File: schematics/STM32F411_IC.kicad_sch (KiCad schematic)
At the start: 24 parts

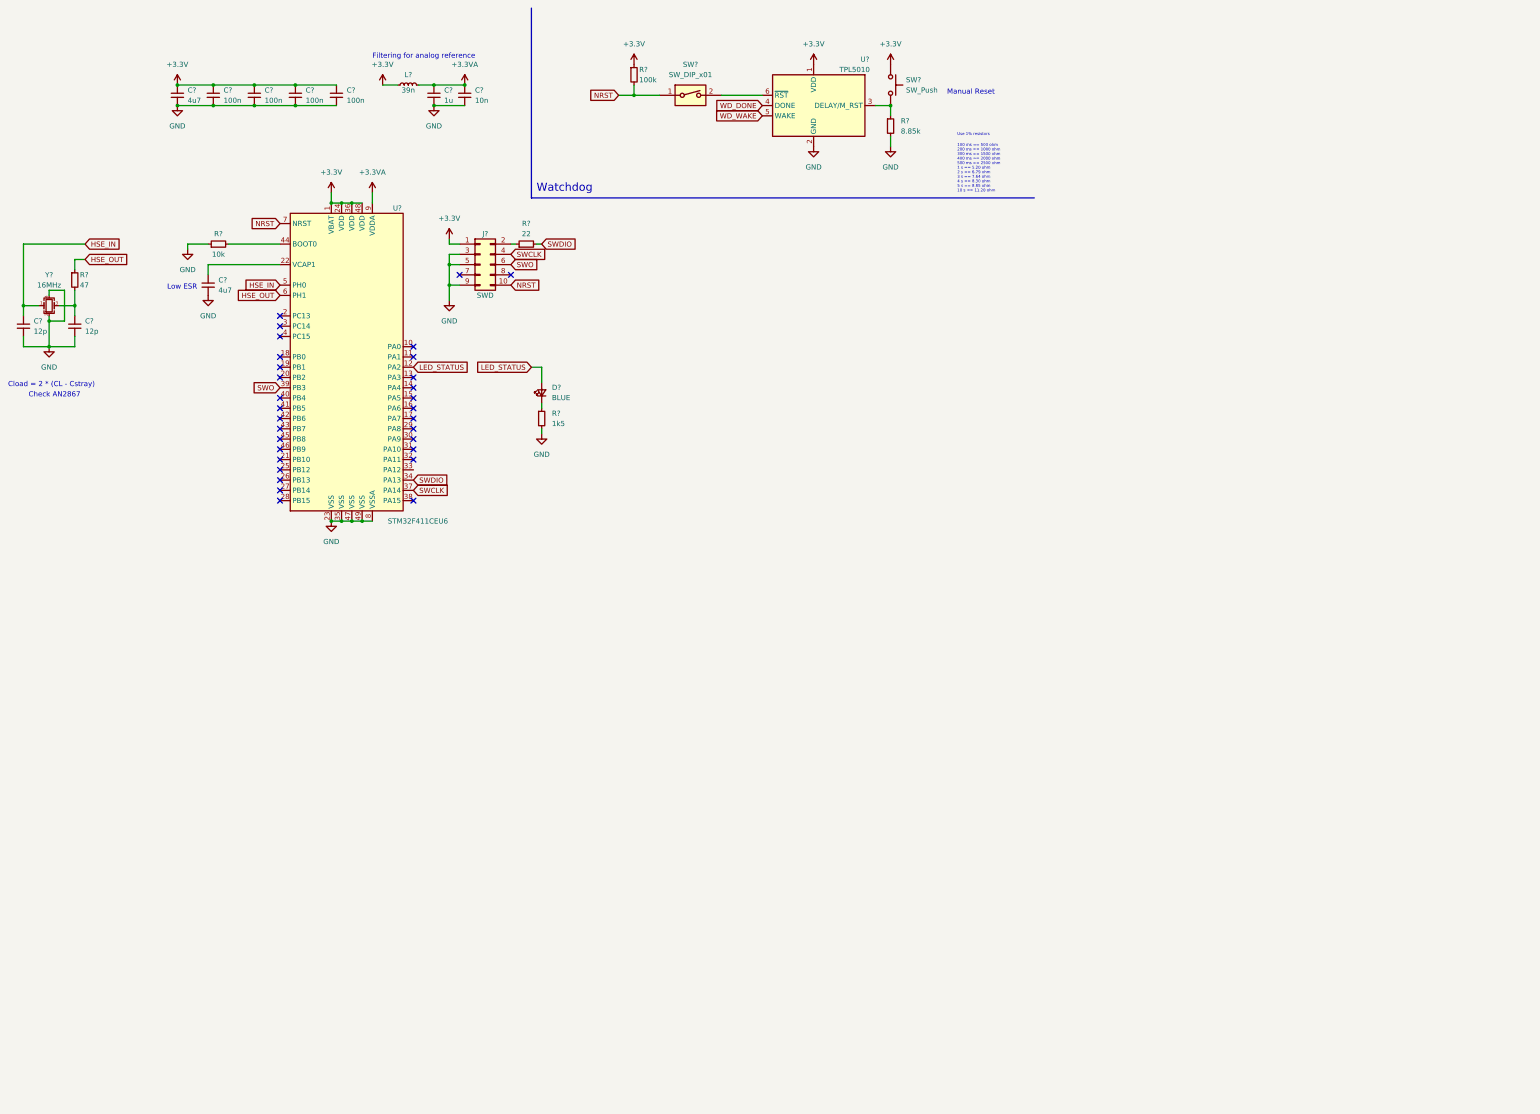
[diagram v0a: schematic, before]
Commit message: Add files via upload
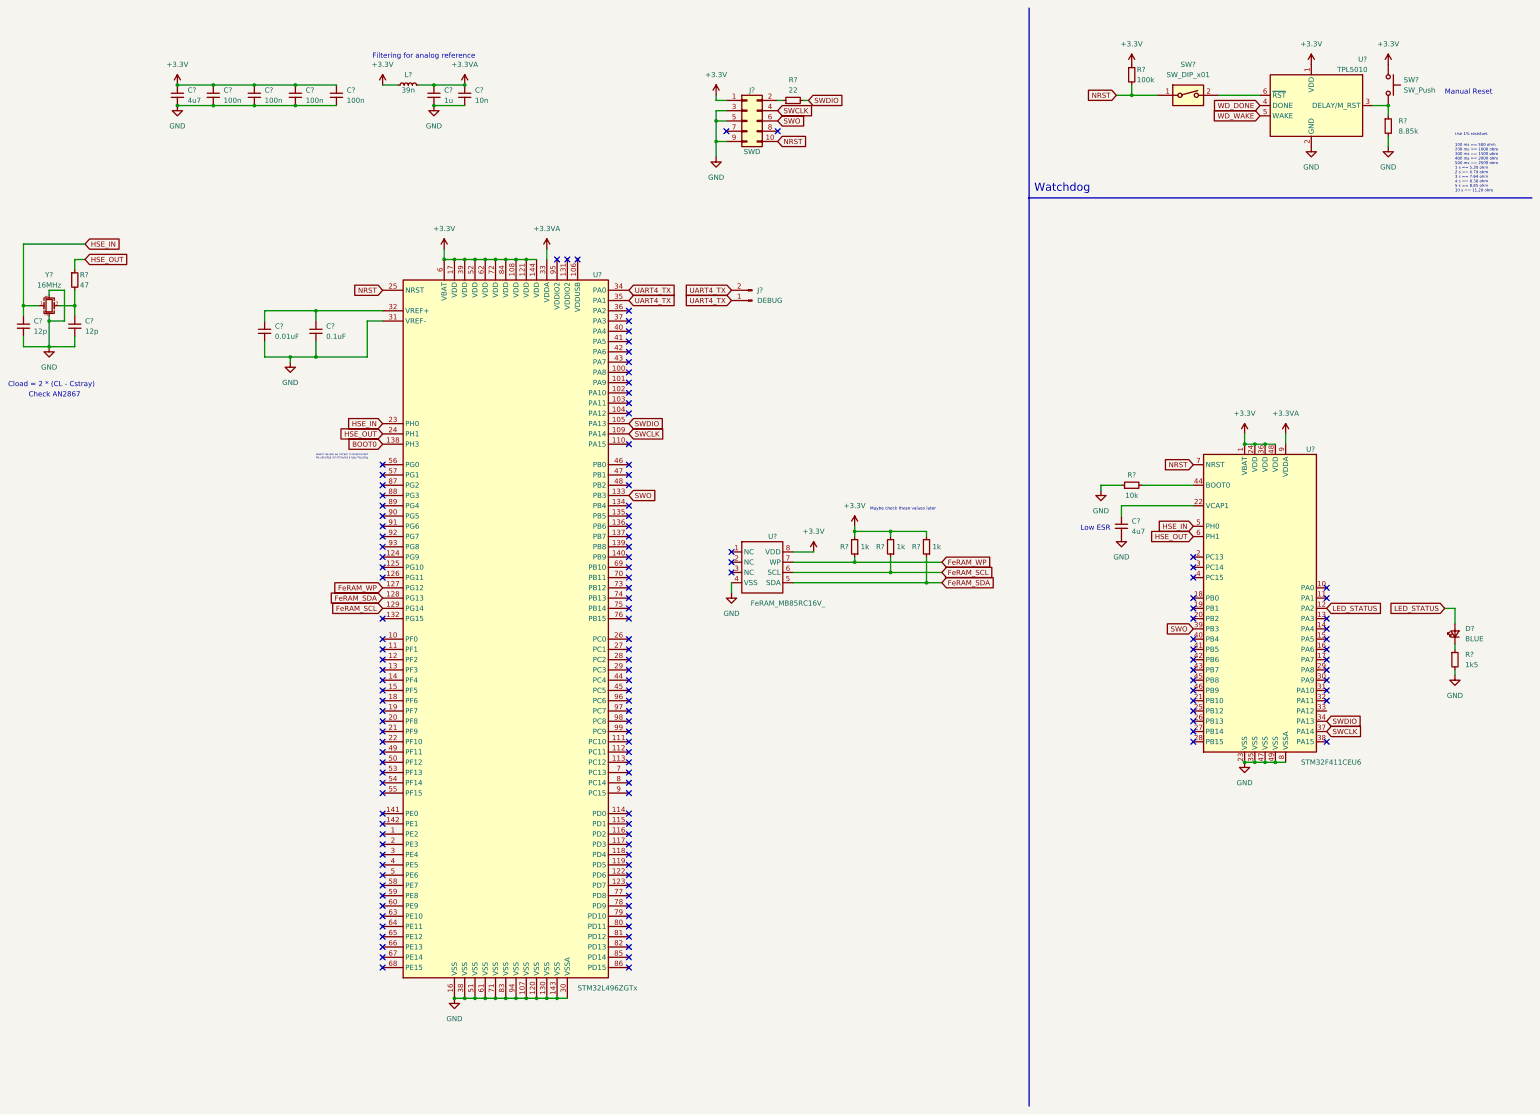
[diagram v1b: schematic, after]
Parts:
- added C?: 0.01uF, symbol Device:C_Small
- added C?: 0.1uF, symbol Device:C_Small
- added J?: DEBUG, symbol Connector:Conn_01x02_Male
- added R? (x3): 1k, symbol Device:R_Small
- added U?: STM32L496ZGTx, Package_QFP:LQFP-144_20x20mm_P0.5mm, symbol MCU_ST_STM32L4:STM32L496ZGTx
- added U?: FeRAM_MB85RC16V_, symbol MyKiCadLibrairy:FeRAM_MB85RC16V_
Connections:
- net +3.3V: now also R?.2, R?.2, R?.2, U?.108 (VDD), U?.121 (VDD), U?.144 (VDD), U?.17 (VDD), U?.39 (VDD), U?.52 (VDD), U?.6 (VBAT), U?.62 (VDD), U?.72 (VDD), U?.8 (VDD), U?.84 (VDD)
- net +3.3VA: now also U?.33 (VDDA)
- net GND: now also C?.2, C?.2, U?.107 (VSS), U?.120 (VSS), U?.130 (VSS), U?.143 (VSS), U?.16 (VSS), U?.30 (VSSA), U?.31 (VREF-), U?.38 (VSS), U?.4 (VSS), U?.51 (VSS), U?.61 (VSS), U?.71 (VSS), U?.83 (VSS), U?.94 (VSS)
- net HSE_IN: now also U?.23 (PH0)
- net HSE_OUT: now also U?.24 (PH1)
- net NRST: now also U?.25 (NRST)
- net SWCLK: now also U?.109 (PA14)
- net SWDIO: now also U?.105 (PA13)
- net SWO: now also U?.133 (PB3)
- new net: C?.1, C?.1, U?.32 (VREF+)
- new net BOOT0: U?.138 (PH3)
- new net FeRAM_SCL: R?.1, U?.129 (PG14), U?.6 (SCL)
- new net FeRAM_SDA: R?.1, U?.128 (PG13), U?.5 (SDA)
- new net FeRAM_WP: R?.1, U?.127 (PG12), U?.7 (WP)
- new net UART4_TX: J?.1 (Pin_1), J?.2 (Pin_2), U?.34 (PA0), U?.35 (PA1)
- no-connect marks 31 -> 141
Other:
- note added: "Avem nevoie sa intram in bootmode? Pe satelitul din filmulet il lasa floating"
- note added: "Maybe check these values later"
- moved on the sheet: C?, D?, J?, R?, SW?, U?
